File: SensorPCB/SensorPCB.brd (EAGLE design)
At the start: 37 x 65 mm, 31 parts, among them T1 33u

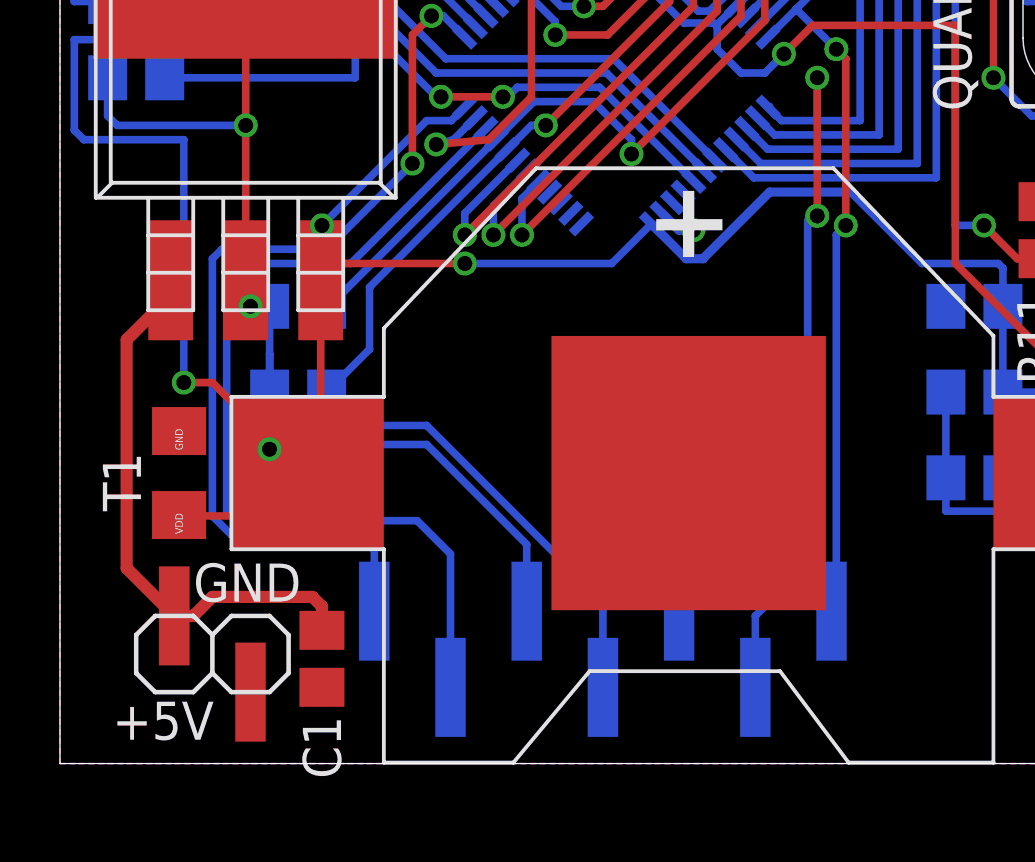
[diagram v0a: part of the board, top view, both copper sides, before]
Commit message: closed #3
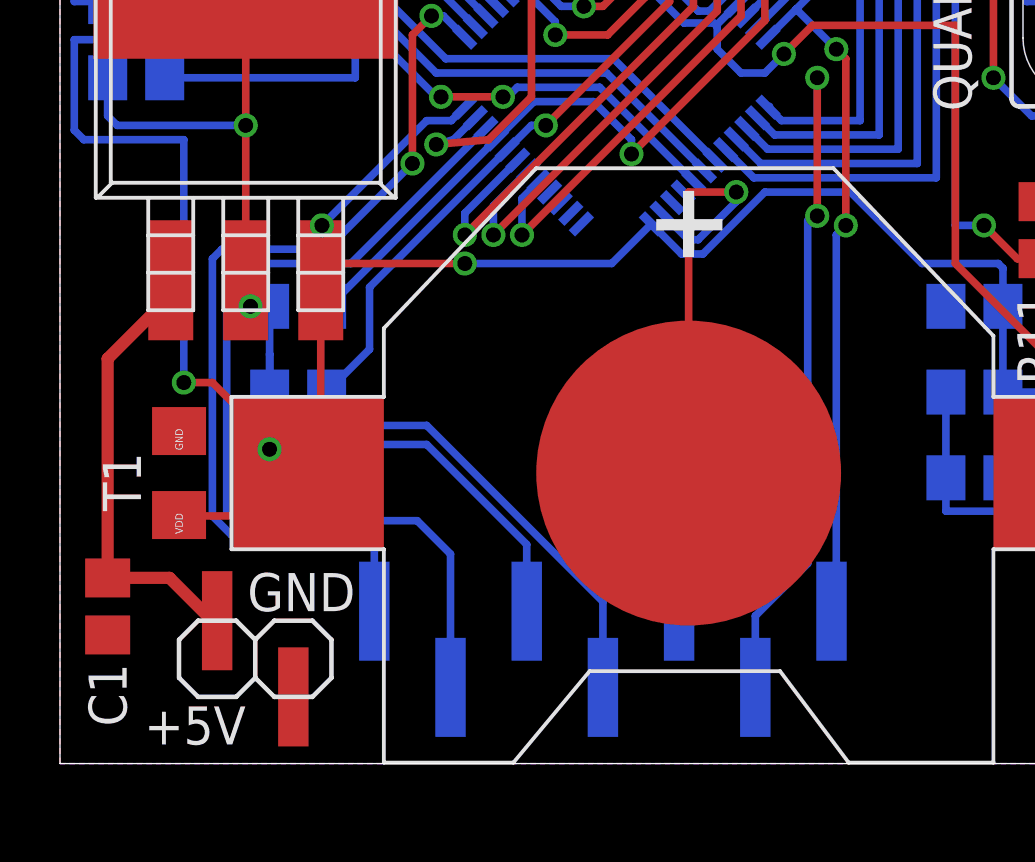
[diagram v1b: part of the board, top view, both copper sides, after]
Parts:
- moved C1 7.35 mm to (1.59, 5.24)
- moved JP1 1.44 mm to (6.51, 3.49)
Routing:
- net GND: track 74.9 -> 88.1 mm
- net +5V: track 19.3 -> 15.5 mm
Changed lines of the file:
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@@
 <layer number="24" name="bOrigins" color="15" fill="1" visible="yes" active="yes"/>
 <layer number="25" name="tNames" color="7" fill="1" visible="yes" active="yes"/>
-<layer number="26" name="bNames" color="7" fill="1" visible="no" active="yes"/>
-<layer number="27" name="tValues" color="7" fill="1" visible="no" active="yes"/>
-<layer number="28" name="bValues" color="7" fill="1" visible="no" active="yes"/>
+<layer number="26" name="bNames" color="7" fill="1" visible="yes" active="yes"/>
+<layer number="27" name="tValues" color="7" fill="1" visible="yes" active="yes"/>
+<layer number="28" name="bValues" color="7" fill="1" visible="yes" active="yes"/>
 <layer number="29" name="tStop" color="7" fill="3" visible="yes" active="yes"/>
 <layer number="30" name="bStop" color="7" fill="6" visible="yes" active="yes"/>
@@
 <dimension x1="0" y1="0" x2="37" y2="0" x3="18.5" y3="-10" textsize="1.778" layer="1"/>
 <dimension x1="37" y1="0" x2="37" y2="65" x3="58.7375" y3="32.5" textsize="1.778" layer="1"/>
-<text x="1.74625" y="0.79375" size="1.27" layer="25">+5V</text>
-<text x="4.445" y="5.3975" size="1.27" layer="25">GND</text>
+<text x="6.19125" y="1.905" size="1.27" layer="25" rot="R180">+5V</text>
+<text x="9.8425" y="6.35" size="1.27" layer="25" rot="R180">GND</text>
 </plain>
 <attributes>
@@
 </autorouter>
 <elements>
-<element name="C1" library="rcl" package="C0805" value="470n" x="8.73125" y="3.4925" smashed="yes" rot="R270">
-<attribute name="NAME" x="8.09625" y="1.5875" size="1.27" layer="25" rot="R270"/>
-<attribute name="VALUE" x="6.19125" y="4.7625" size="1.27" layer="27" rot="R270"/>
+<element name="C1" library="rcl" package="C0805" value="470n" x="1.5875" y="5.23875" smashed="yes" rot="R270">
+<attribute name="NAME" x="0.9525" y="3.33375" size="1.27" layer="25" rot="R270"/>
+<attribute name="VALUE" x="-0.9525" y="6.50875" size="1.27" layer="27" rot="R270"/>
 </element>
 <element name="C10" library="rcl" package="C0805" value="100n" x="34.29" y="27.94" smashed="yes" rot="MR180">
@@
 <attribute name="VALUE" x="4.92125" y="59.3725" size="1.27" layer="27" rot="R270"/>
 </element>
-<element name="JP1" library="pinhead" package="1X02SMD" value="" x="5.08" y="3.65125" smashed="yes">
-<attribute name="VALUE" x="2.54" y="0.47625" size="1.27" layer="27"/>
+<element name="JP1" library="pinhead" package="1X02SMD" value="" x="6.50875" y="3.4925" smashed="yes">
+<attribute name="VALUE" x="3.96875" y="0.3175" size="1.27" layer="27"/>
 </element>
 </elements>
@@
 <vertex x="0" y="0"/>
 </polygon>
-<wire x1="20.066796875" y1="18.343721875" x2="20.63051875" y2="17.78" width="0.3048" layer="16"/>
-<wire x1="20.63051875" y1="17.78" x2="21.11375" y2="17.78" width="0.3048" layer="16"/>
-<wire x1="21.11375" y1="17.78" x2="21.2725" y2="17.78" width="0.3048" layer="16"/>
-<via x="21.11375" y="17.78" extent="1-16" drill="0.5"/>
 <wire x1="12.54125" y1="20.6375" x2="14.2875" y2="20.79625" width="0.254" layer="1"/>
 <wire x1="14.2875" y1="20.79625" x2="15.71625" y2="22.225" width="0.254" layer="1"/>
@@
 <via x="6.19125" y="21.2725" extent="1-16" drill="0.5"/>
 <contactref element="JP1" pad="2"/>
+<wire x1="20.066796875" y1="18.343721875" x2="20.94801875" y2="17.4625" width="0.254" layer="16"/>
+<wire x1="20.94801875" y1="17.4625" x2="21.2725" y2="17.4625" width="0.254" layer="16"/>
+<wire x1="20.955" y1="9.68375" x2="20.955" y2="19.05" width="0.254" layer="1"/>
+<wire x1="20.955" y1="19.05" x2="22.5425" y2="19.05" width="0.254" layer="1"/>
+<via x="22.5425" y="19.05" extent="1-16" drill="0.5"/>
+<wire x1="21.2725" y1="17.4625" x2="22.5425" y2="18.7325" width="0.254" layer="16"/>
+<wire x1="22.5425" y1="18.7325" x2="22.5425" y2="19.05" width="0.254" layer="16"/>
 </signal>
 <signal name="+3V3">
@@
 <wire x1="3.4925" y1="25.08" x2="3.4925" y2="24.13" width="0.254" layer="16"/>
 <wire x1="3.4925" y1="24.13" x2="0.47625" y2="24.13" width="0.254" layer="16"/>
-<wire x1="19.71324375" y1="17.99016875" x2="20.8759125" y2="16.8275" width="0.3048" layer="16"/>
-<wire x1="20.8759125" y1="16.8275" x2="21.43125" y2="16.8275" width="0.3048" layer="16"/>
-<wire x1="21.43125" y1="16.8275" x2="23.65375" y2="19.05" width="0.3048" layer="16"/>
-<wire x1="23.65375" y1="19.05" x2="26.3525" y2="19.05" width="0.3048" layer="16"/>
 <wire x1="17.379790625" y1="28.101796875" x2="20.79625" y2="24.6853375" width="0.254" layer="16"/>
 <wire x1="21.874553125" y1="24.60625" x2="21.795465625" y2="24.6853375" width="0.254" layer="16"/>
@@
 <wire x1="6.985" y1="10.4775" x2="7.14375" y2="10.63625" width="0.254" layer="16"/>
 <wire x1="7.14375" y1="10.63625" x2="12.22375" y2="10.63625" width="0.254" layer="16"/>
+<wire x1="19.71324375" y1="17.99016875" x2="20.7171625" y2="16.98625" width="0.254" layer="16"/>
+<wire x1="20.7171625" y1="16.98625" x2="21.43125" y2="16.98625" width="0.254" layer="16"/>
+<wire x1="21.43125" y1="16.98625" x2="23.495" y2="19.05" width="0.254" layer="16"/>
+<wire x1="23.495" y1="19.05" x2="26.3525" y2="19.05" width="0.254" layer="16"/>
 </signal>
 <signal name="+5V">
 <contactref element="LM3940" pad="1"/>
 <contactref element="C1" pad="1"/>
-<wire x1="2.2225" y1="6.50875" x2="2.2225" y2="14.12875" width="0.4064" layer="1"/>
 <wire x1="4.1675" y1="16.07375" x2="3.69125" y2="16.11" width="0.4064" layer="1"/>
-<wire x1="2.2225" y1="14.12875" x2="3.69125" y2="15.5975" width="0.4064" layer="1"/>
+<wire x1="1.5875" y1="13.49375" x2="3.69125" y2="15.5975" width="0.4064" layer="1"/>
 <wire x1="3.69125" y1="15.5975" x2="3.69125" y2="16.11" width="0.4064" layer="1"/>
 <contactref element="JP1" pad="1"/>
-<wire x1="3.81" y1="4.92125" x2="2.2225" y2="6.50875" width="0.4064" layer="1"/>
-<wire x1="3.81" y1="4.92125" x2="3.96875" y2="5.08" width="0.4064" layer="1"/>
-<wire x1="8.73125" y1="4.4425" x2="8.73125" y2="5.23875" width="0.4064" layer="1"/>
-<wire x1="8.73125" y1="5.23875" x2="8.41375" y2="5.55625" width="0.4064" layer="1"/>
-<wire x1="8.41375" y1="5.55625" x2="5.08" y2="5.55625" width="0.4064" layer="1"/>
-<wire x1="5.08" y1="5.55625" x2="4.445" y2="4.92125" width="0.4064" layer="1"/>
-<wire x1="4.445" y1="4.92125" x2="3.81" y2="4.92125" width="0.4064" layer="1"/>
+<wire x1="1.5875" y1="13.49375" x2="1.5875" y2="6.18875" width="0.4064" layer="1"/>
+<wire x1="1.5875" y1="6.18875" x2="1.59" y2="6.19125" width="0.4064" layer="1"/>
+<wire x1="1.59" y1="6.19125" x2="3.65125" y2="6.19125" width="0.4064" layer="1"/>
+<wire x1="3.65125" y1="6.19125" x2="5.08" y2="4.7625" width="0.4064" layer="1"/>
+<wire x1="5.08" y1="4.7625" x2="5.23875" y2="4.7625" width="0.4064" layer="1"/>
 </signal>
 <signal name="SWCLK">
@@
 <wire x1="29.845" y1="29.845" x2="29.845" y2="17.93875" width="0.254" layer="16"/>
 <wire x1="30.7975" y1="17.93875" x2="29.845" y2="17.93875" width="0.254" layer="16"/>
-<wire x1="29.845" y1="17.93875" x2="30.7975" y2="17.93875" width="0" layer="19" extent="1-16"/>
 <wire x1="30.7975" y1="17.93875" x2="31.90875" y2="16.8275" width="0.254" layer="1"/>
 <wire x1="31.90875" y1="16.8275" x2="32.385" y2="16.8275" width="0.254" layer="1"/>
